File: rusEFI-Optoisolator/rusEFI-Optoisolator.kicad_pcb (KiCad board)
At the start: 2 copper layers, 43.2 x 12.7 mm, 11 parts, among them J1 Conn_01x02_Male, J2 Conn_01x03_Male, U1 4N25

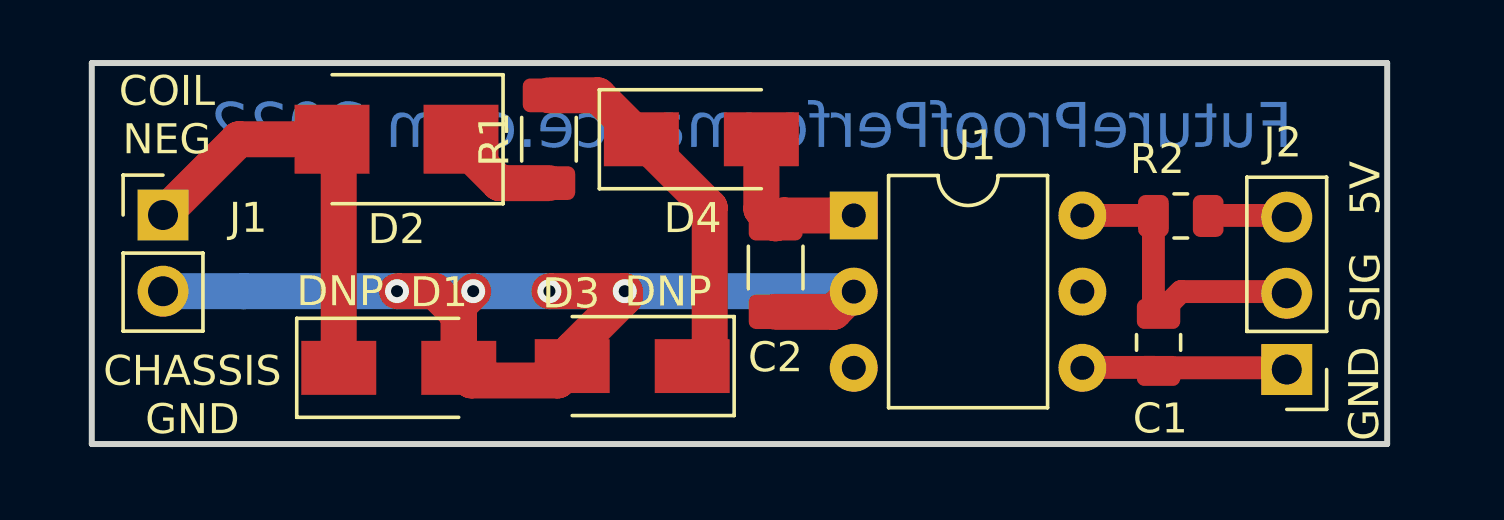
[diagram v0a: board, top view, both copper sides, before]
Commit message: New version
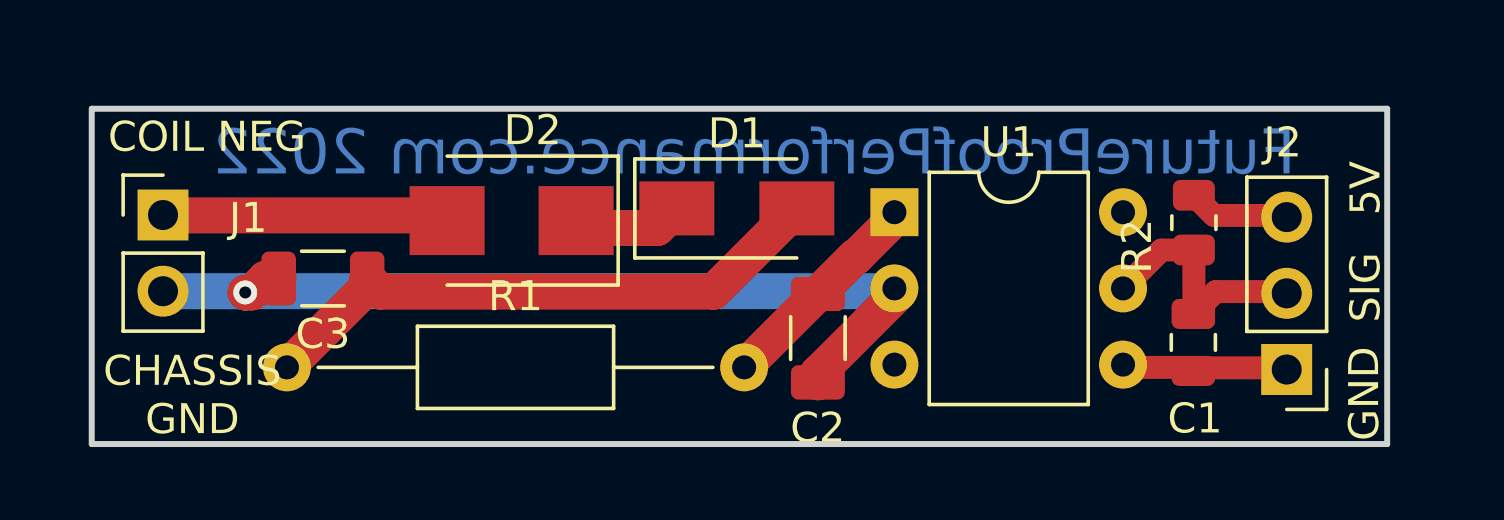
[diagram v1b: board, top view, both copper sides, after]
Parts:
- removed D3: DNP, Diode_SMD:D_SMA
- removed D4: 1SMA4748A, Diode_SMD:D_SMA
- added C3: 0.2uF, Capacitor_SMD:C_1206_3216Metric, F.Cu at (124.5, 85.9)
- C2: value 0.0022uF1 -> 0.001uF
- D1: value DNP -> 1SMA4748A
- R1: footprint Resistor_SMD:R_1206_3216Metric -> Resistor_THT:R_Axial_DIN0207_L6.3mm_D2.5mm_P15.24mm_Horizontal
- moved D1 12.5 mm to (138.3, 83.6)
- moved R1 11.6 mm to (123.3, 88.9), turned to 0 degrees
- moved D2 4.70 mm to (130.8, 84.0)
- moved C2 2.74 mm to (141.0, 87.9)
- moved U1 1.36 mm to (143.6, 83.7)
- moved C1 1.16 mm to (153.6, 88.1)
- moved R2 0.49 mm to (153.6, 84.1), turned to 90 degrees
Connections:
- D1 pad 1: Coil_in -> Net-(D2-Pad1)
- D1 pad 2: GND -> Net-(C3-Pad1)
- R1 pad 1: Net-(D2-Pad1) -> Net-(C3-Pad1)
- R1 pad 2: Net-(D3-Pad1) -> Net-(C2-Pad1)
- U1 pad 5: unconnected-(U1-Pad5) -> Trigger_Output
- U1 pad 6: Trigger_Output -> unconnected-(U1-Pad6)
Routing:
- net Net-(C3-Pad1): track 0.00 -> 19.7 mm
- net GND: track 43.2 -> 29.9 mm, vias 4 -> 1
- net Net-(D3-Pad1): track 12.4 -> 0.00 mm
- net Coil_in: track 14.4 -> 9.55 mm
- net Trigger_Output: track 10.3 -> 8.47 mm
- net Net-(C2-Pad1): track 5.71 -> 7.28 mm
- net Net-(C1-Pad2): track 6.93 -> 5.61 mm
- net 5V: track 2.65 -> 3.40 mm
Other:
- board size 43.2 x 12.7 mm -> 43.2 x 11.2 mm
- board text added: "Optoisolator for rusEFI"
